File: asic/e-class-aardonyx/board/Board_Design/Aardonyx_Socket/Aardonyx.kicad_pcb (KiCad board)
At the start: 4 copper layers, 329 parts, among them J1 Conn_1x4, J10 Conn_1x3_M, J11 Conn_1x8, J12 Conn_1x3_M, J13 USB_B_6PIN, J14 Conn_1x4, J15 Conn_1x3_M, J16 USB_OTG, J17 Conn_1x8, J18 Conn_1x3_M, J19 Conn_1x3_M, J2 Conn_1x6, J3 Conn_1x10_F, J4 Conn_1x8_F, J5 Conn_1x8_F, J6 Conn_1x6_F, J7 Conn_1x3_M, J8 PJ-202H PWRJACK, J9 Conn_1x6, Q1 FDN339AN, SW1 FSM2JSMAATR, SW2 SW_DIP_x03, SW3 SW_SPST, U1 LSF0108PWR, U10 ADM1186, U11 FT2232H, U12 TPS7A7002DDAR, U13 TPS54627DDAR, U14 93LC56BT-I_OT, U15 TPS7A7002DDAR, U2 SKT32E, U3 IS42S32160F-TSOP2, U4 LSF0108PWR, U5 CDCE913PW, U6 ADC128S102CIMTX/NOPB, U7 74AUP1G09GW, U8 IS25LP256x-xM, U9 CAT24M01WI-GT3, Y1 27MHz, Y2 12MHz

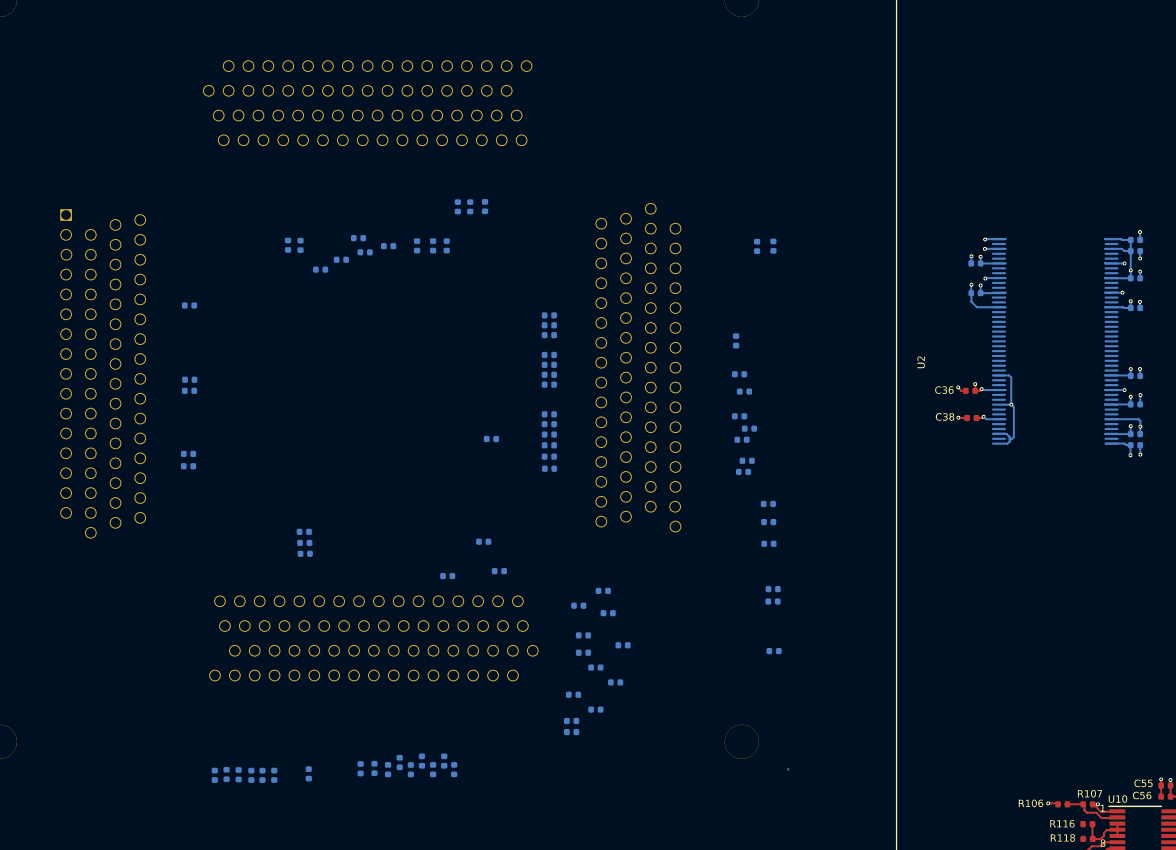
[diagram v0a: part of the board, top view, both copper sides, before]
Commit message: update sock track & foot prin soc th
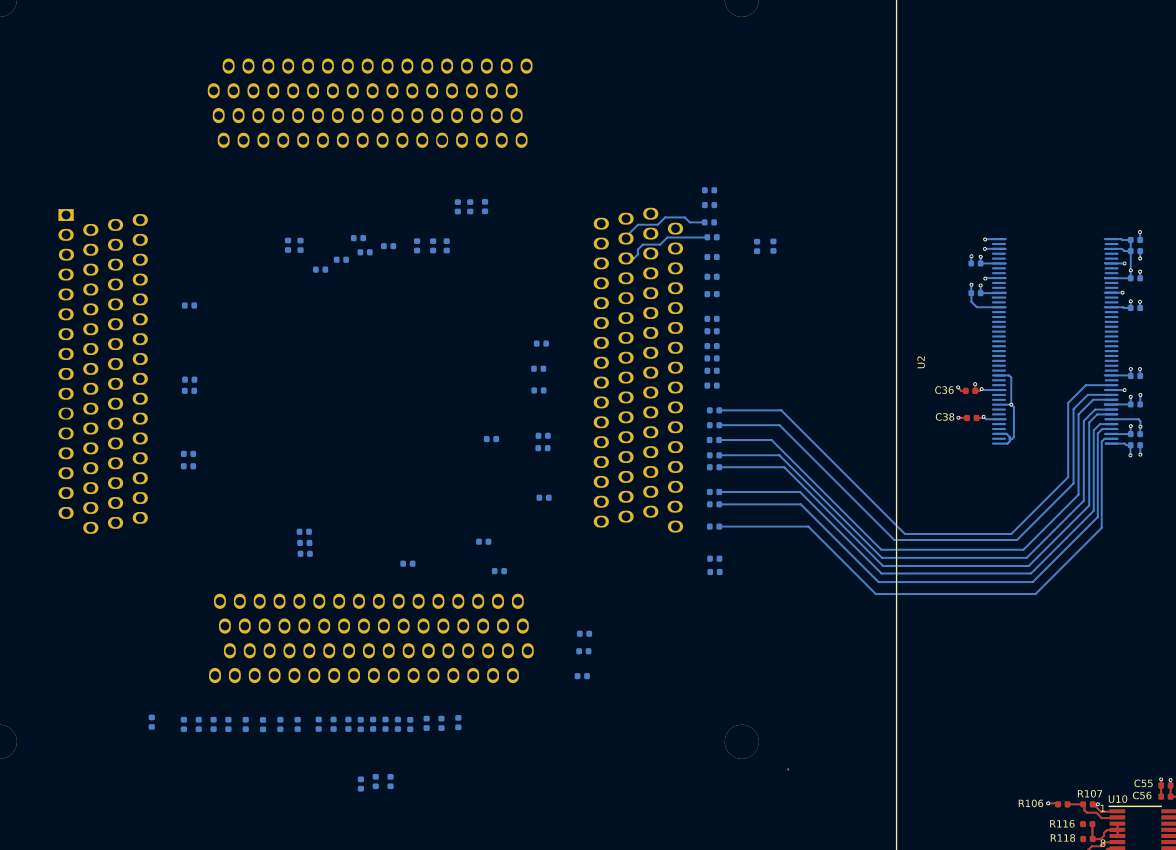
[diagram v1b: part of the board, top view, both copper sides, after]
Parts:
- moved R77 34.2 mm to (122.9, 112.3), turned to 270 degrees
- moved R76 29.9 mm to (124.6, 112.2), turned to 270 degrees
- moved C34 28.5 mm to (151.5, 73.1)
- moved C13 28.4 mm to (151.7, 89.0)
- moved C25 28.4 mm to (151.6, 82.6)
- moved C33 28.4 mm to (151.2, 75.7)
- moved C20 28.4 mm to (151.6, 83.9)
- moved C30 28.4 mm to (151.2, 77.9)
- moved R73 28.1 mm to (126.4, 112.2), turned to 270 degrees
- moved R66 27.5 mm to (169.3, 96.6), turned to 180 degrees
- moved R78 21.5 mm to (138.0, 112.2), turned to 270 degrees
- moved R22 21.5 mm to (168.7, 57.4)
- moved R26 20.6 mm to (169.0, 62.2)
- moved R25 20.1 mm to (168.7, 60.7)
- moved R27 20.0 mm to (169.0, 64.2)
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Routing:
- net /sdram/SDRAM_D16: track 0.00 -> 56.9 mm
- net /sdram/SDRAM_D18: track 0.00 -> 56.7 mm
- net /sdram/SDRAM_D20: track 0.00 -> 56.5 mm
- net /sdram/SDRAM_D17: track 0.00 -> 56.4 mm
- net /sdram/SDRAM_D19: track 0.00 -> 56.3 mm
- net /sdram/SDRAM_D22: track 0.00 -> 55.7 mm
- net /sdram/SDRAM_D23: track 0.00 -> 55.5 mm
- net /sdram/SDRAM_D21: track 0.00 -> 55.5 mm
- net Net-(R26-Pad2): track 0.00 -> 9.53 mm
- net Net-(R25-Pad2): track 0.00 -> 9.29 mm
